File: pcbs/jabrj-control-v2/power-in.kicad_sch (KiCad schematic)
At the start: 10 parts, among them J301 43045-0201, U301 TVS2701DRBR, U302 TPS26600RHFR

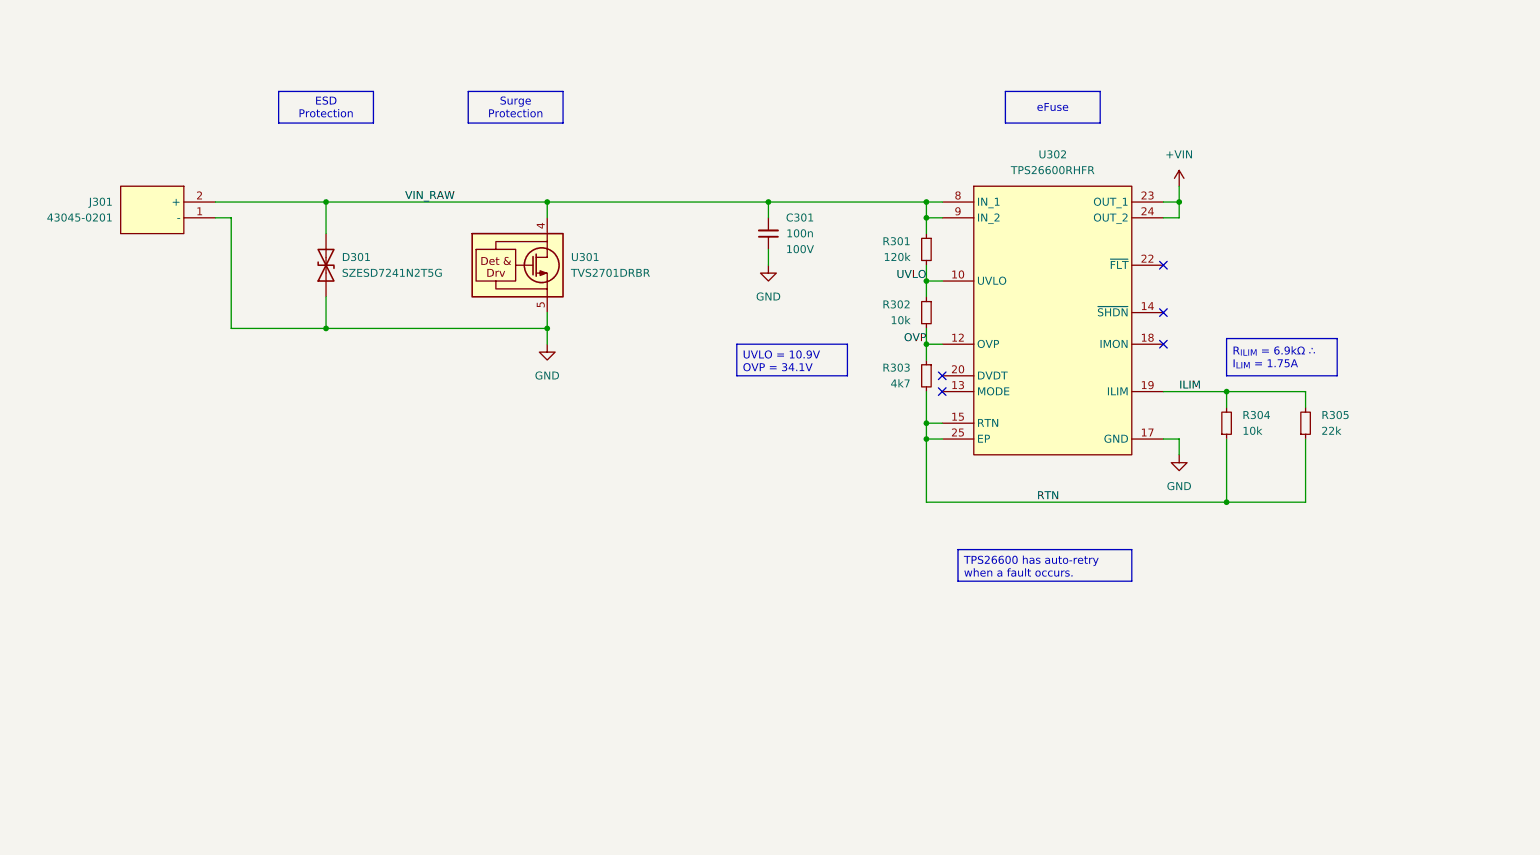
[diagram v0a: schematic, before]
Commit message: 603 Unrouted
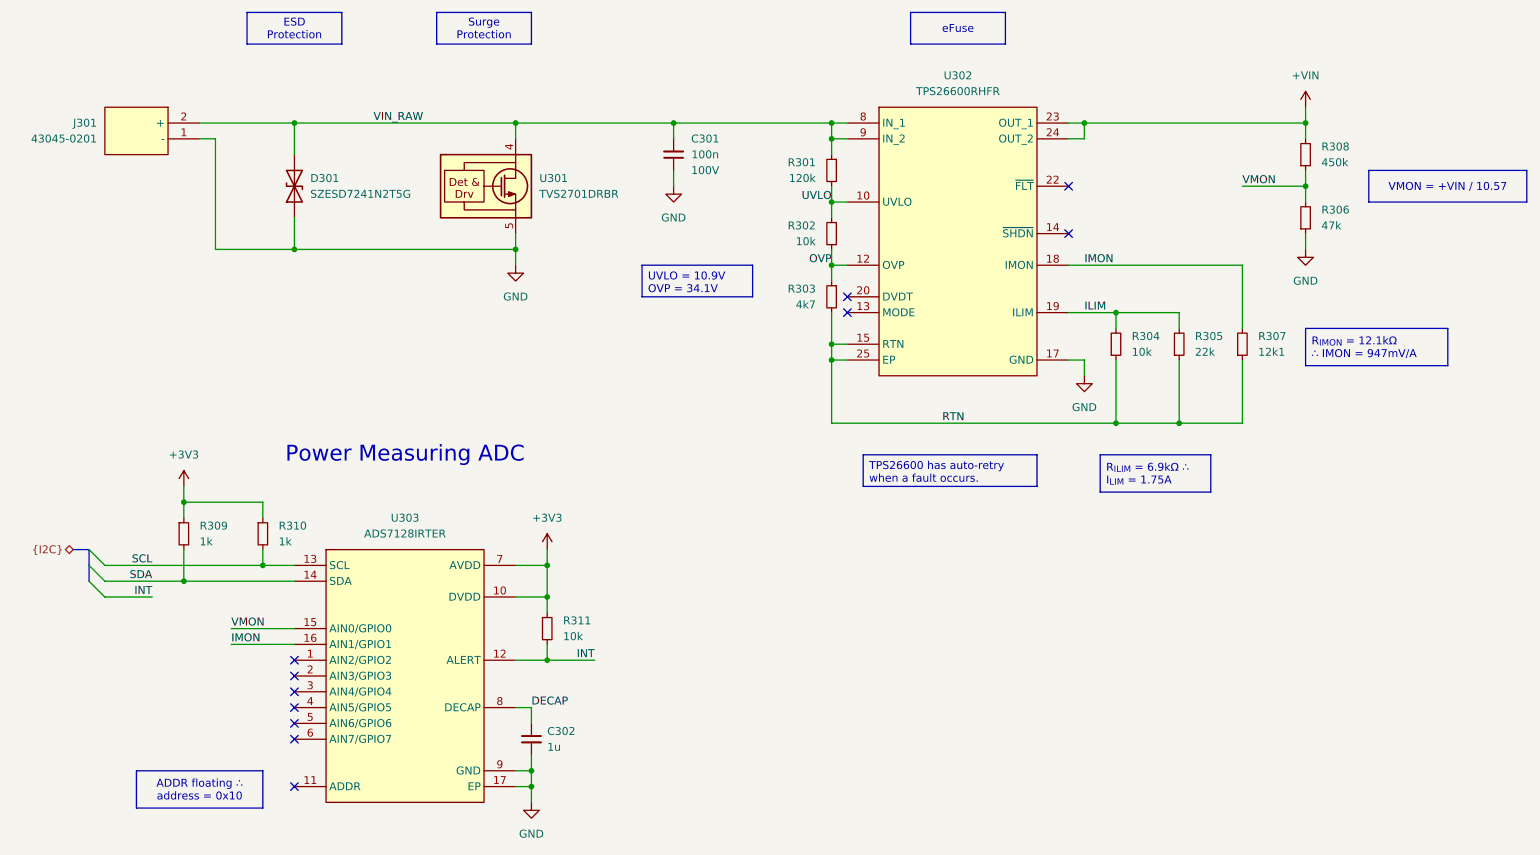
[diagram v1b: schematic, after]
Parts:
- added C302: 1u, project_footprints:C_0402, symbol DEV:C_SMALL
- added R306: 47k, project_footprints:R_0402, symbol Device:R_Small
- added R307: 12k1, project_footprints:R_0402, symbol Device:R_Small
- added R308: 450k, project_footprints:R_0402, symbol Device:R_Small
- added R309, R310: 1k, project_footprints:R_0402, symbol DEV:R_SMALL
- added R311: 10k, project_footprints:R_0402, symbol DEV:R_SMALL
- added U303: ADS7128IRTER, project_footprints:QFN50P300X300X80-17N-D, symbol ADC:ADS7128IRTER
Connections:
- net +VIN: now also R308.2
- net GND: now also C302.2, R306.1, U303.17 (EP), U303.9 (GND)
- net RTN: now also R307.1
- net IMON: now reaches U302.18 (IMON)
- net IMON: now also R307.2, U303.16 (AIN1/GPIO1)
- new net +3V3: R309.1, R310.1, R311.1, U303.10 (DVDD), U303.7 (AVDD)
- new net DECAP: C302.1, U303.8 (DECAP)
- new net INT: R311.2, U303.12 (ALERT)
- new net SCL: R310.2, U303.13 (SCL)
- new net SDA: R309.2, U303.14 (SDA)
- new net VMON: R306.2, R308.1, U303.15 (AIN0/GPIO0)
- no-connect marks 5 -> 11
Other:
- note added: "Power Measuring ADC"
- moved on the sheet: C301, D301, J301, R301, R302, R303, R304, R305, U301, U302
